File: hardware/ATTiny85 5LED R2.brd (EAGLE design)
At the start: 22.5 x 91.4 mm, 9 parts, among them U1 TINY85-20-DIP

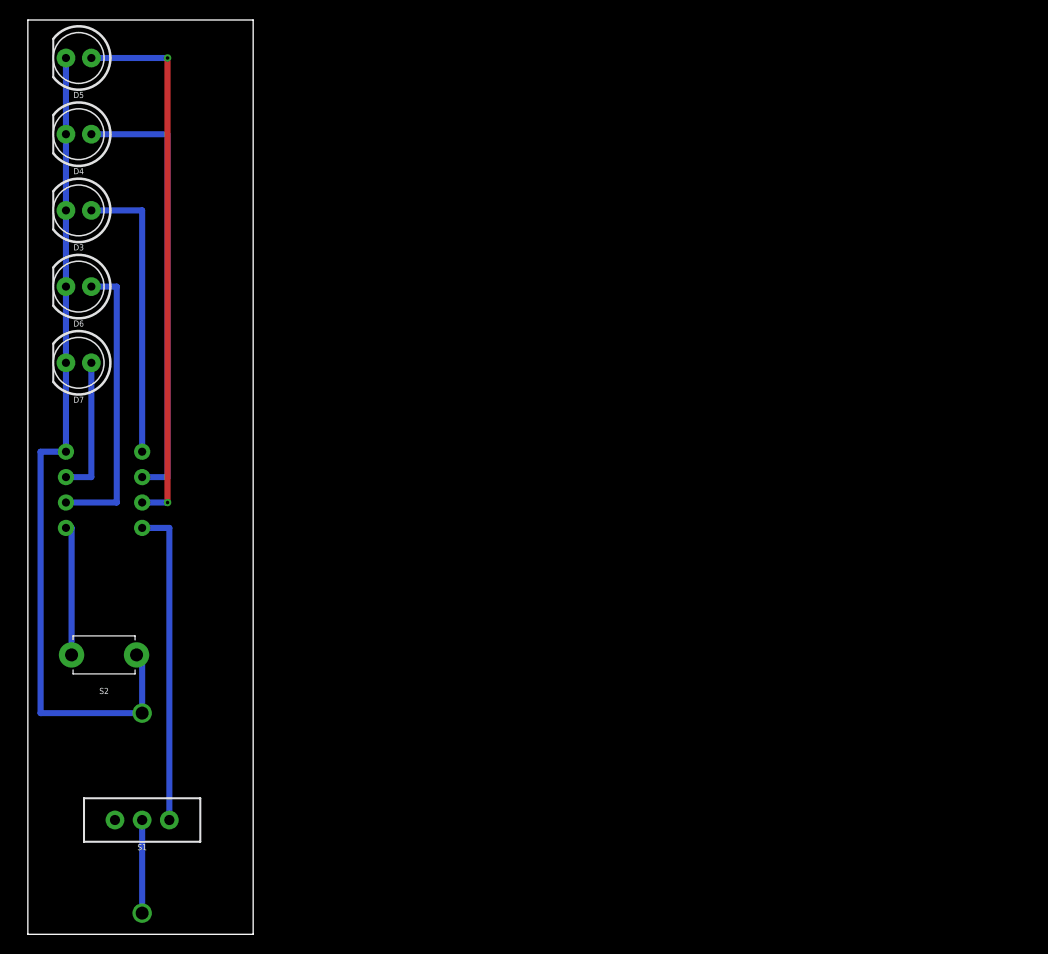
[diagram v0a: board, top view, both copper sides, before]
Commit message: updating eagle files
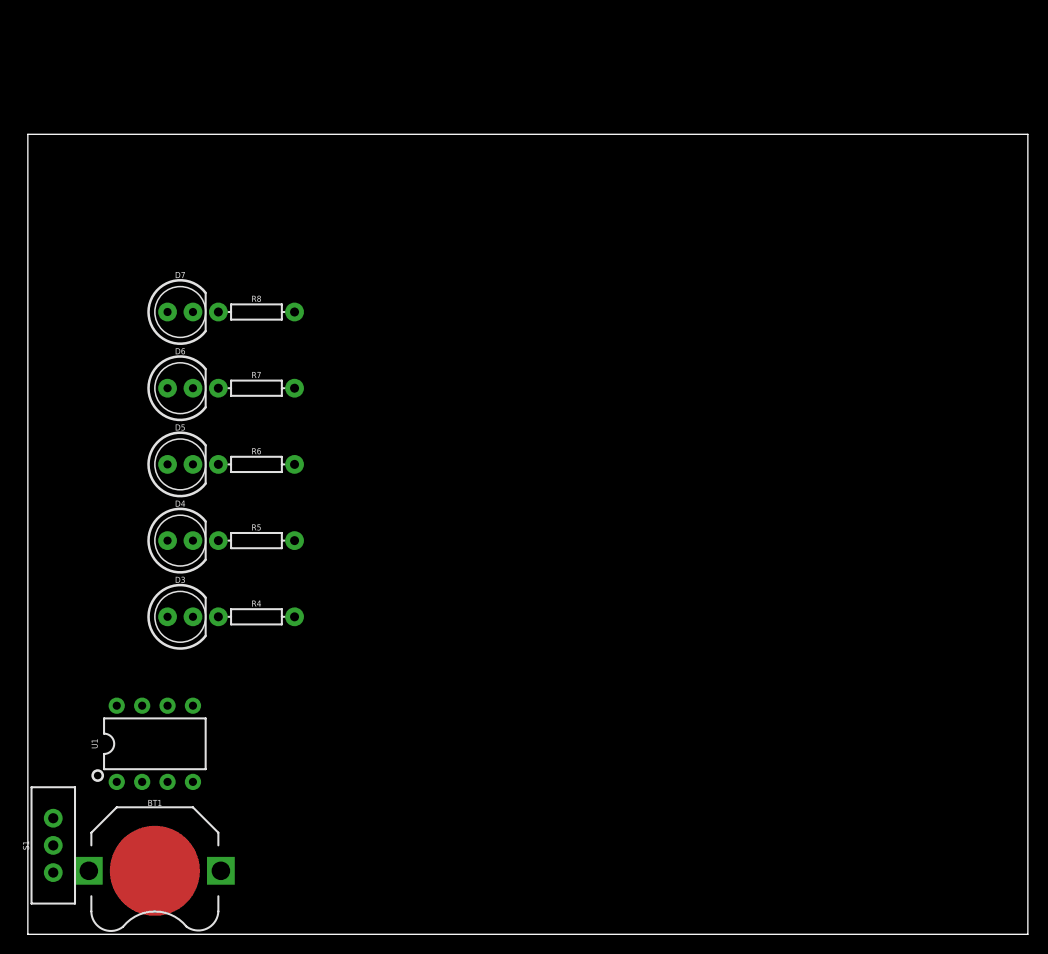
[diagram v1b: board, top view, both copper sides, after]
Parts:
- removed S2: (no value), adafruit:TACT_PANA-EVQ
- added R4, R5, R6, R7, R8: 1k, SparkFun-Resistors:AXIAL-0.3
- BT1: device SparkFun-Batteries:BATTCOM_20MM_PTH -> SparkFun-Batteries:BATTCON_12MM_PTH
- moved D4 41.9 mm to (15.2, 39.4), turned to 0 degrees
- moved D3 41.9 mm to (15.2, 31.8), turned to 0 degrees
- moved D5 41.9 mm to (15.2, 47.0), turned to 0 degrees
- moved U1 25.9 mm to (12.7, 19.1), flipped to the top, turned to 0 degrees
- moved D6 14.4 mm to (15.2, 54.6), turned to 0 degrees
- moved D7 11.4 mm to (15.2, 62.2), turned to 0 degrees
- moved S1 9.25 mm to (2.54, 8.89), turned to 0 degrees
- moved BT1 7.73 mm to (12.7, 6.35), flipped to the top, turned to 180 degrees
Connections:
- new net N$3: D3.K, R4.P$1
- new net N$4: D4.K, R5.P$1
- new net N$5: D5.K, R6.P$1
- new net N$6: D6.K, R7.P$1
- new net N$7: D7.K, R8.P$1
- net GND: now also BT1.GND, R4.P$2, R5.P$2, R6.P$2, R7.P$2, R8.P$2; no longer BT1.2, D3.K, D4.K, D5.K, D6.K, D7.K, S2.P$1
- net N$1: now also BT1.VCC@1, S1.3; no longer BT1.1, S1.2
- net PB5: no longer S2.P$2
- net VCC: now also S1.2; no longer S1.3
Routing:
- net GND: track 84.6 -> 0.00 mm
- net PB2: track 54.6 -> 0.00 mm, vias 2 -> 0
- net PB1: track 44.5 -> 0.00 mm
- net VCC: track 31.9 -> 0.00 mm
- net PB0: track 29.2 -> 0.00 mm
- net PB3: track 29.2 -> 0.00 mm
- net PB4: track 14.0 -> 0.00 mm
- net PB5: track 13.3 -> 0.00 mm
- net N$1: track 9.31 -> 0.00 mm
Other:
- board size 22.5 x 91.4 mm -> 100 x 80 mm
